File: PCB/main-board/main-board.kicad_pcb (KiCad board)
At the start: 2 copper layers, 25 x 23.7 mm, 43 parts, among them J1 USB-C 16P (12V + CAN/I2C), J2 Motor (JST-PH 2P), U1 ESP32-S3-SuperMini, U2 DRV8876RGTR, U3 MLX90393SLW-ABA-011-RE, U4 AP63205WU-7, U5 SN65HVD230

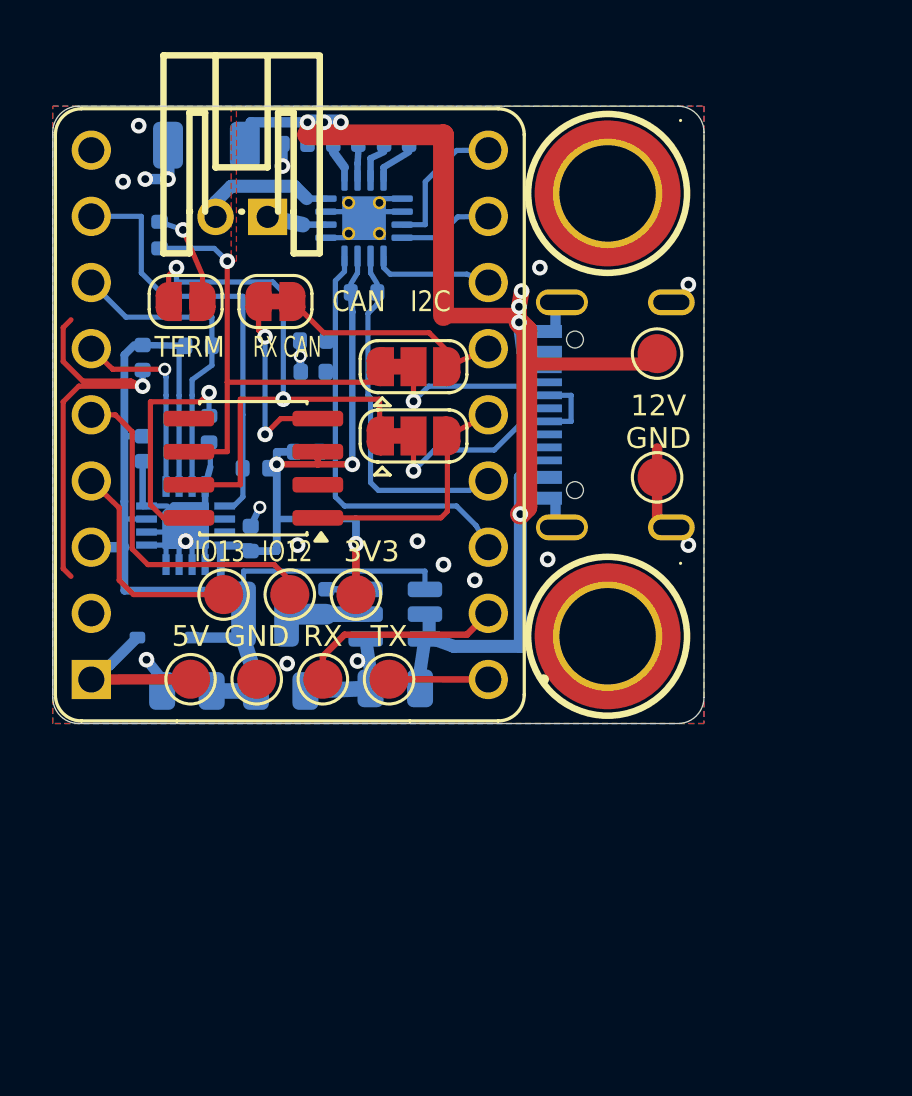
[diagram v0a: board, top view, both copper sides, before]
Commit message: PCB dev
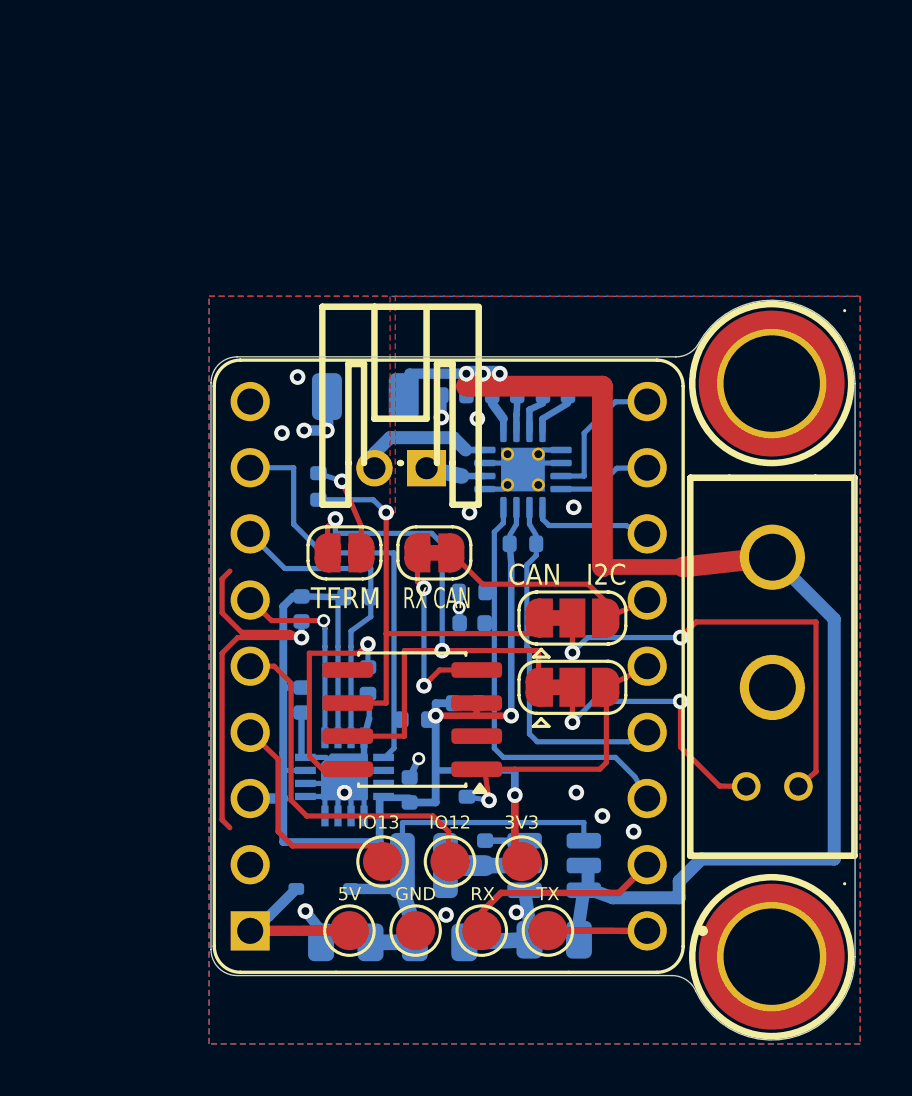
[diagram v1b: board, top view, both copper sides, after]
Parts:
- removed J1: USB-C 16P (12V + CAN/I2C), main-board:USB-C_HX-TYPE-C-16PIN_NPTH-pegs
- removed TP8, TP9: Pad, TestPoint:TestPoint_Pad_D1.5mm
- added CN2: XT30APB, main-board:CONN-TH_XT30APB, F.Cu at (39.6, 33.7)
- added R7: 10k, Resistor_SMD:R_0402_1005Metric, B.Cu at (27.9, 38.0)
- moved H2 13.8 mm to (39.6, 44.6)
- moved TP5 12.1 mm to (30.0, 41.0)
- moved TP1 12.0 mm to (27.2, 41.0)
- moved TP2 11.9 mm to (24.7, 41.0)
- moved C11 11.4 mm to (21.6, 31.3)
- moved C12 11.4 mm to (28.1, 31.9)
- moved C13 11.4 mm to (27.9, 34.9)
- moved C7 11.4 mm to (29.4, 23.1)
- moved C8 11.4 mm to (31.3, 23.1)
- moved R2 11.4 mm to (30.1, 28.8)
- moved C1 11.4 mm to (31.2, 44.0)
- moved C2 11.4 mm to (28.6, 40.7)
- moved C3 11.4 mm to (26.9, 44.1)
- moved C4 11.4 mm to (23.2, 44.1)
- moved C5 11.4 mm to (27.4, 23.1)
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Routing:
- net /BUS_N: track 9.67 -> 17.8 mm, vias 1 -> 2
- net GND: track 44.0 -> 38.9 mm, vias 20 -> 18
- net /SDA_CANTX: track 9.74 -> 11.7 mm, vias 0 -> 1
- net /BUS_P: track 8.90 -> 10.7 mm, vias 1 -> 2
- net +12V: track 53.5 -> 52.5 mm, vias 7 -> 3
- net /MAG_SDA: track 16.9 -> 16.2 mm
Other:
- board size 25 x 23.7 mm -> 24.7 x 28.4 mm
